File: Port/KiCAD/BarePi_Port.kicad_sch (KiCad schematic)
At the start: 14 parts, among them J1 IN, J10 SPI1, J11 PORT, J12 UART, J2 OUT, J3 WCH-LINK, J4 I2C, J5 I2C, J6 I2C, J7 SPI0, J8 SPI1, J9 SPI0, U1 CH32V002A4M6

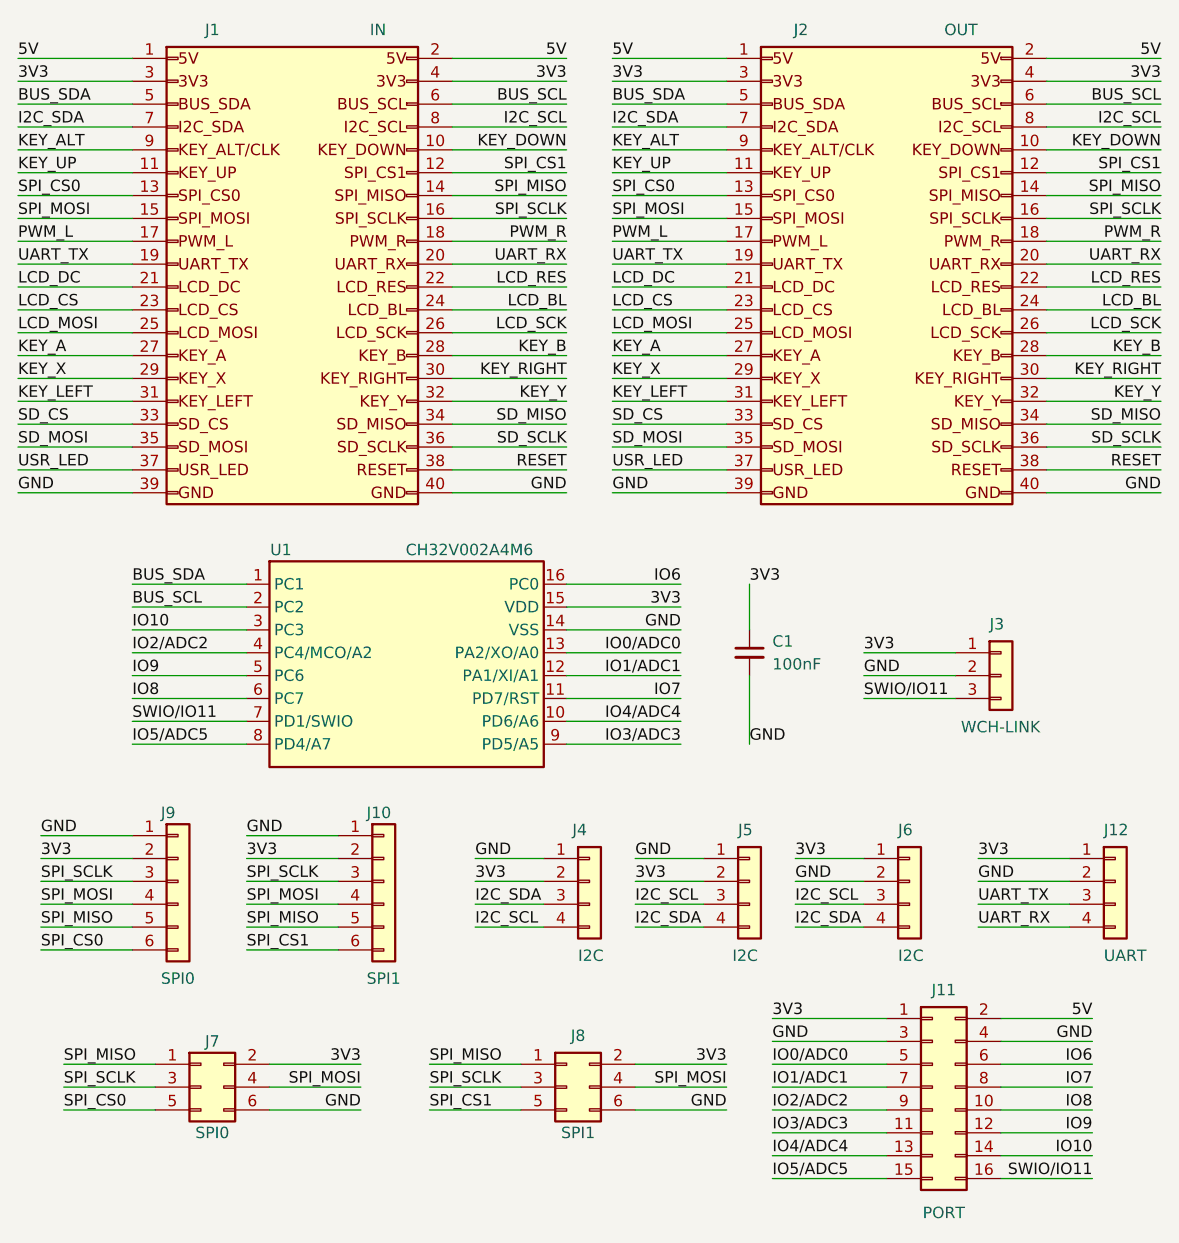
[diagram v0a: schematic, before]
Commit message: init
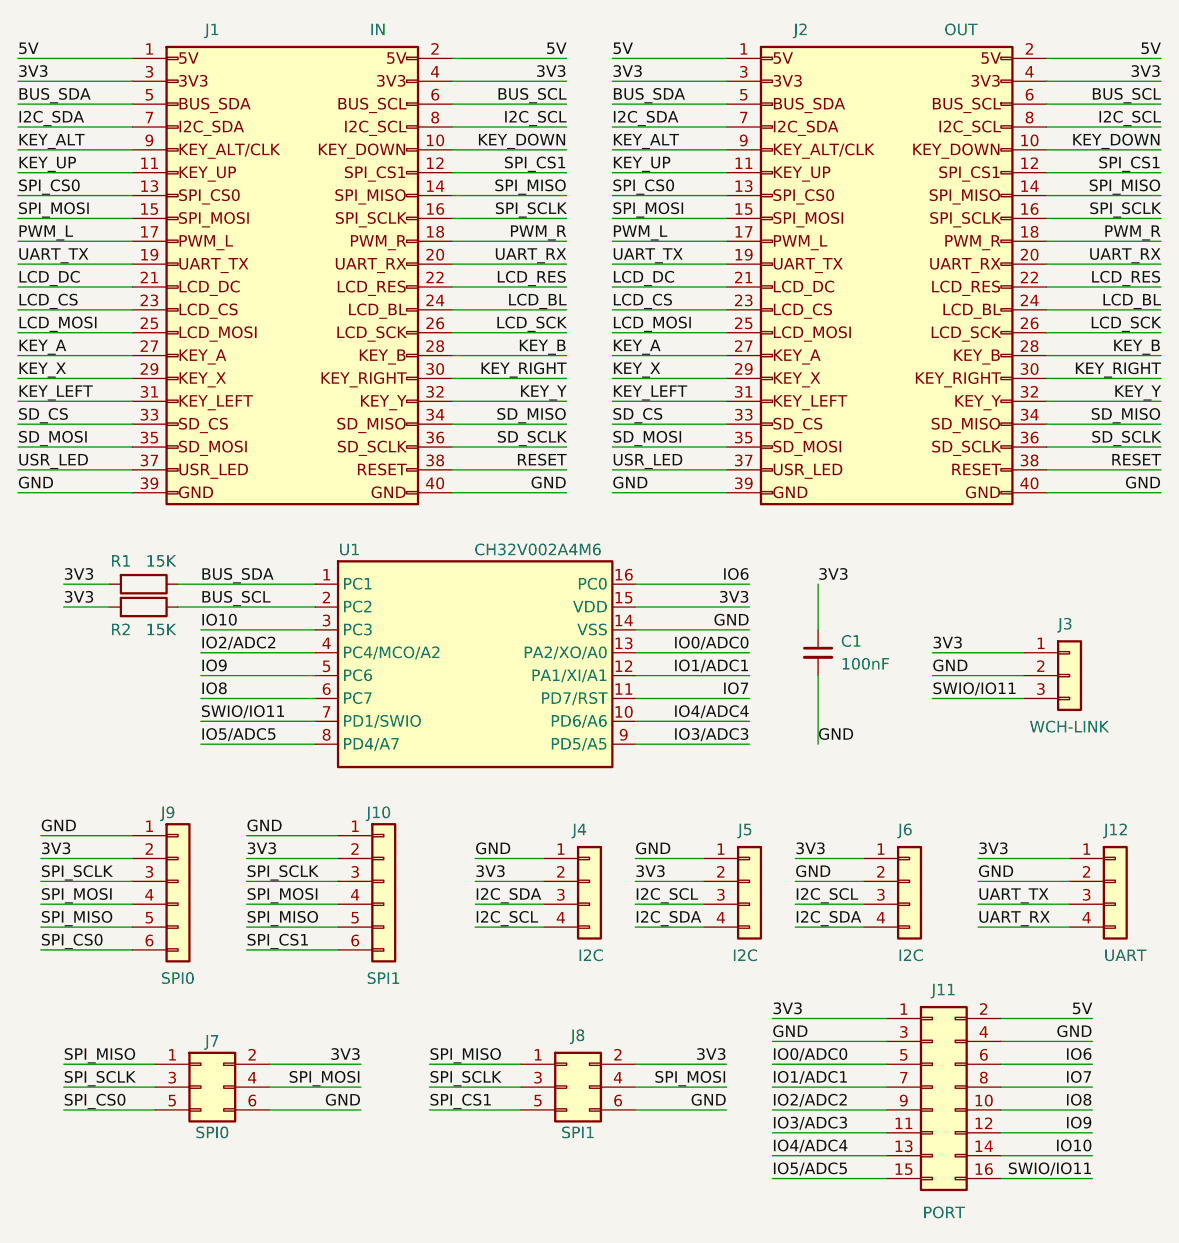
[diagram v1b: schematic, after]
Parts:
- added R1, R2: 15K, Resistor_SMD:R_1206_3216Metric_Pad1.30x1.75mm_HandSolder, symbol Device:R
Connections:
- net 3V3: now also R1.2, R2.2
- net BUS_SCL: now also R2.1
- net BUS_SDA: now also R1.1
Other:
- moved on the sheet: C1, J3, U1
